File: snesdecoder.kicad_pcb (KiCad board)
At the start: 2 copper layers, 19.2 x 17.6 mm, 12 parts, among them J1 SNES Controller Input, J2 Power, J3 12PAD, U1 74HC04, U2 74LS161, U3 TLC6C5912, U4 74LVC1G08

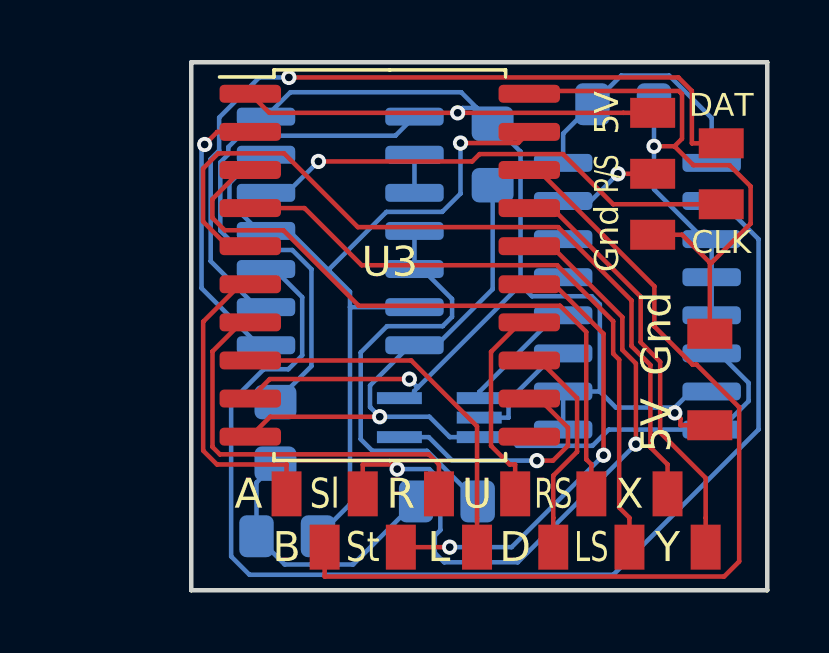
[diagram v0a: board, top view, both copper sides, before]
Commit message: snesdecoder compact release
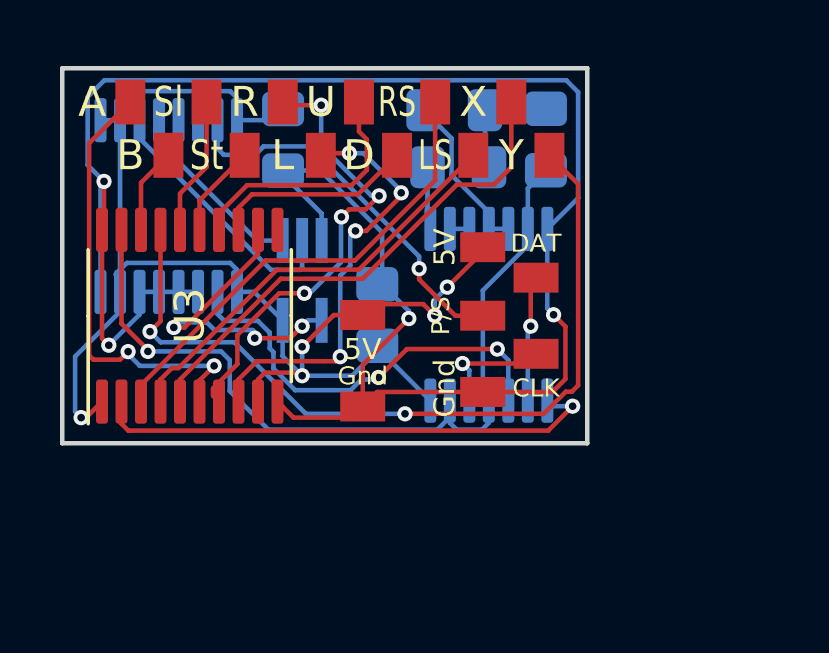
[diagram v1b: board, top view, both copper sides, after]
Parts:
- U1: footprint Package_SO:SOIC-14_3.9x8.7mm_P1.27mm -> Package_SO:TSSOP-14_4.4x5mm_P0.65mm
- U2: footprint Package_SO:SOIC-16_3.9x9.9mm_P1.27mm -> Package_SO:TSSOP-16_4.4x5mm_P0.65mm
- U3: footprint Package_SO:SOIC-20W_7.5x12.8mm_P1.27mm -> Package_SO:TSSOP-20_4.4x6.5mm_P0.65mm
- moved U2 15.9 mm to (154.1, 81.6), turned to 90 degrees
- moved R2 15.8 mm to (166.6, 79.4), turned to 90 degrees
- moved J3 14.1 mm to (159.0, 78.8)
- moved J2 13.6 mm to (159.5, 86.8), turned to 90 degrees
- moved C1 13.0 mm to (163.6, 78.4), turned to 0 degrees
- moved C2 10.8 mm to (161.0, 85.2), turned to 270 degrees
- moved R1 10.7 mm to (163.7, 80.3), turned to 0 degrees
- moved C3 7.00 mm to (157.9, 79.4)
- moved J1 7.00 mm to (163.5, 85.2)
- moved U3 6.88 mm to (154.8, 85.2), turned to 90 degrees
- moved U4 6.47 mm to (158.5, 84.1), turned to 270 degrees
- moved U1 5.69 mm to (164.7, 85.2), turned to 270 degrees
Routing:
- net Net-(J3-Pad2): track 31.2 -> 2.86 mm
- net Net-(U1-Pad10): track 40.0 -> 14.2 mm, vias 0 -> 2
- net Net-(J1-Pad4): track 26.6 -> 4.21 mm
- net +5V: track 64.5 -> 45.4 mm, vias 3 -> 5
- net Net-(J3-Pad3): track 23.3 -> 4.63 mm, vias 2 -> 0
- net Net-(R1-Pad1): track 18.0 -> 2.46 mm
- net Net-(J3-Pad12): track 14.2 -> 27.4 mm, vias 0 -> 2
- net Net-(J1-Pad2): track 16.4 -> 3.92 mm
- net Net-(J3-Pad4): track 15.2 -> 3.11 mm, vias 2 -> 0
- net Net-(J3-Pad11): track 27.1 -> 16.9 mm
- net GND: track 58.1 -> 67.9 mm, vias 2 -> 4
- net Net-(J1-Pad3): track 3.36 -> 12.8 mm
- net Net-(C1-Pad1): track 14.7 -> 5.51 mm
- net Net-(U1-Pad8): track 9.46 -> 17.1 mm
- net Net-(J3-Pad10): track 21.4 -> 14.3 mm
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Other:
- board size 19.2 x 17.6 mm -> 17.5 x 12.5 mm
